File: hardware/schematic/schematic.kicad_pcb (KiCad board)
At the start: 2 copper layers, 23 parts, among them J1 Conn_01x09_Pin, J2 Conn_01x09_Pin, J3 ADS1115, J4 PE_SENSE_1, J5 N_TEST, J6 PE_SENSE_0, J7 PE_FORCE_IN, J8 PE_FORCE_OUT, J9 L_TEST, Q1 Q_NMOS_GSD, U1 LM317

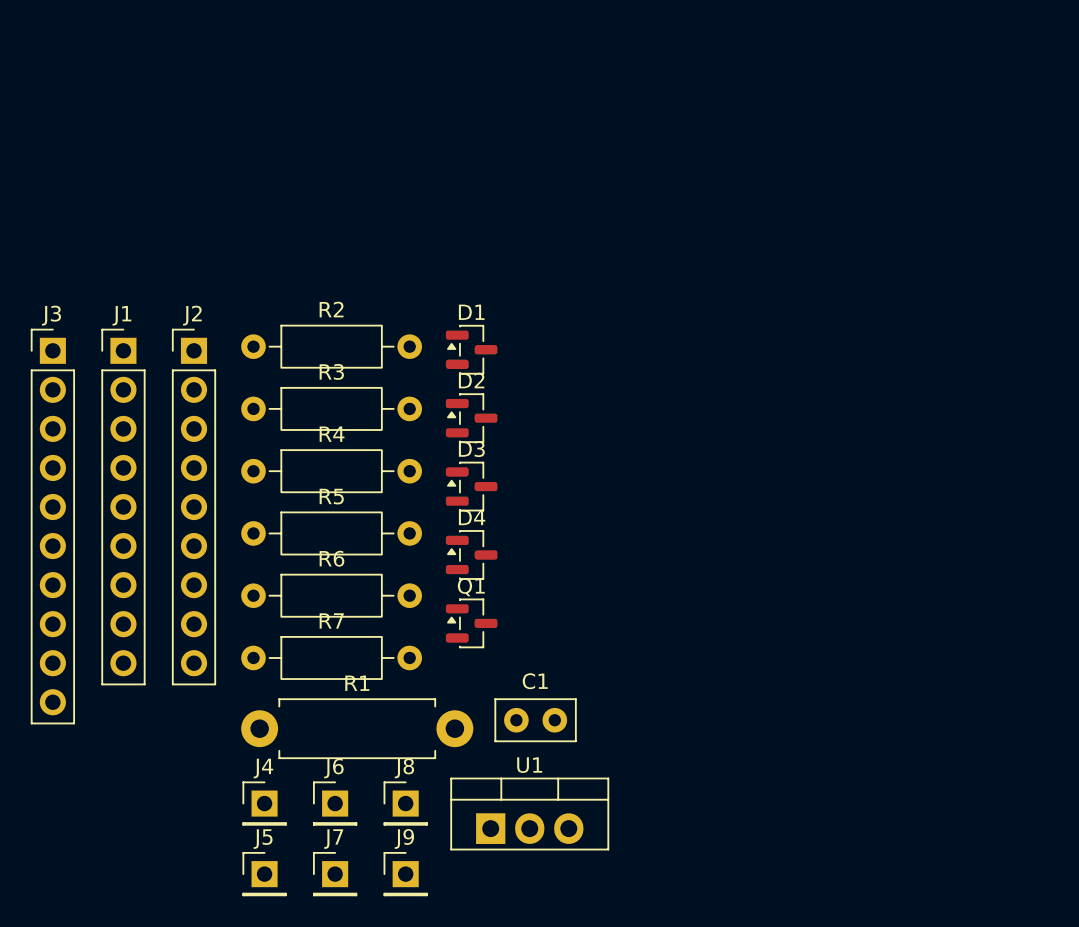
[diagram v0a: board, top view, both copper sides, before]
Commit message: update
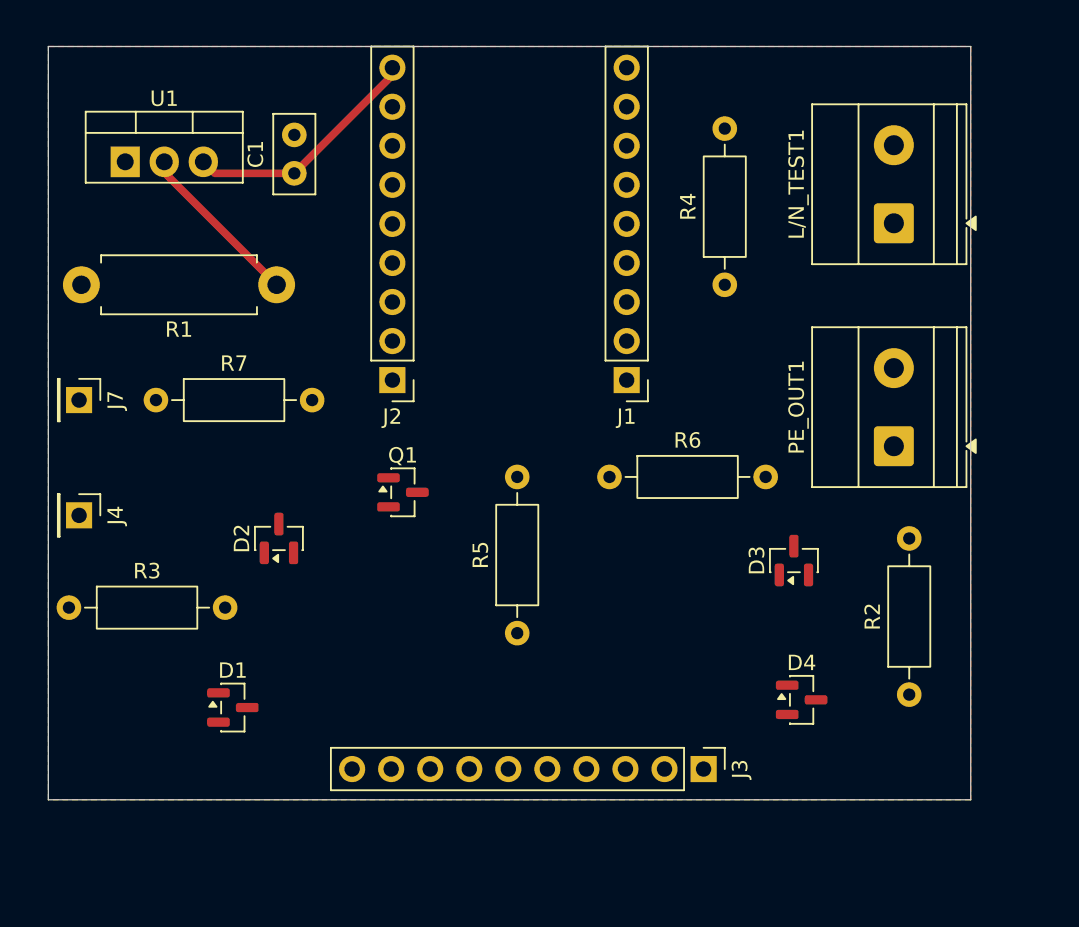
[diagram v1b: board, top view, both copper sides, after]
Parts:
- removed J5: N_TEST, Connector_PinHeader_2.54mm:PinHeader_1x01_P2.54mm_Vertical
- removed J6: PE_SENSE_0, Connector_PinHeader_2.54mm:PinHeader_1x01_P2.54mm_Vertical
- removed J8: PE_FORCE_OUT, Connector_PinHeader_2.54mm:PinHeader_1x01_P2.54mm_Vertical
- removed J9: L_TEST, Connector_PinHeader_2.54mm:PinHeader_1x01_P2.54mm_Vertical
- added L/N_TEST1: Conn_01x02, TerminalBlock_Phoenix:TerminalBlock_Phoenix_MKDS-1,5-2-5.08_1x02_P5.08mm_Horizontal, F.Cu at (142.5, 111.5)
- added PE_OUT1: Conn_01x02, TerminalBlock_Phoenix:TerminalBlock_Phoenix_MKDS-1,5-2-5.08_1x02_P5.08mm_Horizontal, F.Cu at (142.5, 126.0)
- moved J3 50.3 mm to (130.1, 147.0), turned to -90 degrees
- moved U1 49.5 mm to (92.5, 107.5)
- moved R2 48.3 mm to (143.5, 142.2), turned to 90 degrees
- moved C1 38.4 mm to (103.5, 108.2), turned to 90 degrees
- moved J7 35.0 mm to (89.5, 123.0), turned to -90 degrees
- moved R4 33.0 mm to (131.5, 115.5), turned to 90 degrees
- moved J1 32.8 mm to (125.1, 121.7), turned to 180 degrees
- moved R1 28.9 mm to (102.3, 115.5), turned to 180 degrees
- moved D1 28.0 mm to (99.5, 143.0)
- moved R6 24.4 mm to (124.0, 128.0)
- moved D4 23.4 mm to (136.5, 142.5)
- moved J4 22.3 mm to (89.5, 130.5), turned to -90 degrees
- moved D3 21.5 mm to (136.0, 133.4), turned to 90 degrees
- moved R5 18.3 mm to (118.0, 138.2), turned to 90 degrees
- moved R7 17.9 mm to (94.5, 123.0)
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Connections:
- net /<NO NET> renamed +5V
- net Net-(J5-Pin_1) renamed /N_TEST
- J2 pad 8: /GND -> GNDREF
- J3 pad 6: /GND -> GNDREF
- J3 pad 9: /GND -> GNDREF
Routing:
- net +5V: track 0.00 -> 15.7 mm
- net Net-(U1-VO): track 0.00 -> 11.0 mm
- added copper zone on F.Cu, net GNDREF
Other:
- board outline added: 60 x 49 mm

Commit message: update
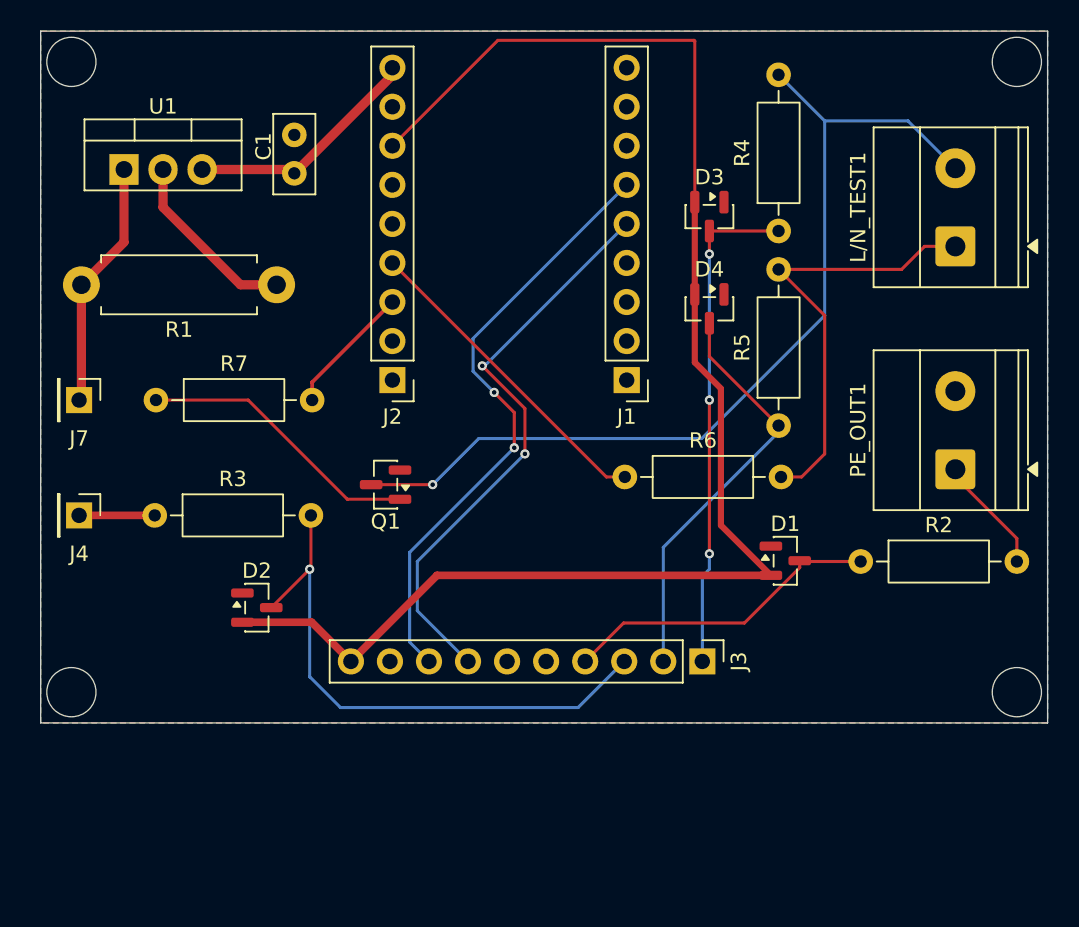
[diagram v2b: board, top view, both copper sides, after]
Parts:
- added REF**: MountingHole_3.2mm_M3, MountingHole:MountingHole_3.2mm_M3, F.Cu at (89.0, 101.0)
- added REF**: MountingHole_3.2mm_M3, MountingHole:MountingHole_3.2mm_M3, F.Cu at (150.5, 101.0)
- added REF**: MountingHole_3.2mm_M3, MountingHole:MountingHole_3.2mm_M3, F.Cu at (89.0, 142.0)
- added REF**: MountingHole_3.2mm_M3, MountingHole:MountingHole_3.2mm_M3, F.Cu at (150.5, 142.0)
- moved D1 37.2 mm to (135.4, 133.4)
- moved D4 26.1 mm to (130.5, 117.1), turned to -90 degrees
- moved D3 23.0 mm to (130.5, 111.1), turned to -90 degrees
- moved R5 21.7 mm to (135.0, 124.7)
- moved R2 9.22 mm to (140.3, 133.5), turned to 0 degrees
- moved R3 8.19 mm to (94.4, 130.5)
- moved J3 7.00 mm to (130.0, 140.0)
- moved R4 4.95 mm to (135.0, 112.0)
- moved D2 4.72 mm to (101.1, 136.5), turned to 0 degrees
- moved L/N_TEST1 4.27 mm to (146.5, 113.0)
- moved PE_OUT1 4.27 mm to (146.5, 127.5)
- moved Q1 1.23 mm to (109.4, 128.5), turned to 180 degrees
- moved R6 1.00 mm to (125.0, 128.0)
- moved U1 0.51 mm to (92.4, 108.0)
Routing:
- net /3V3: track 0.00 -> 97.1 mm
- net /N_TEST: track 0.00 -> 60.7 mm, vias 0 -> 1
- net /I2C_SCL: track 0.00 -> 39.6 mm, vias 0 -> 2
- net /I2C_SDA: track 0.00 -> 37.9 mm, vias 0 -> 2
- net /PE_TEST_RE: track 0.00 -> 36.7 mm, vias 0 -> 1
- net /N_T: track 0.00 -> 32.7 mm, vias 0 -> 3
- net Net-(L/N_TEST1-Pin_1): track 0.00 -> 28.8 mm
- net /L_T: track 0.00 -> 26.6 mm
- net /PE_TEST: track 0.00 -> 20.9 mm
- net /GP27: track 0.00 -> 20.9 mm
- net Net-(Q1-G): track 0.00 -> 18.5 mm
- net Net-(J7-Pin_1): track 0.00 -> 16.2 mm
- net /GP26: track 0.00 -> 8.54 mm
- net Net-(PE_OUT1-Pin_1): track 0.00 -> 7.66 mm
- net Net-(J4-Pin_1): track 0.00 -> 4.92 mm
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- added copper zone on B.Cu, net GNDREF
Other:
- board size 60 x 49 mm -> 65.5 x 45 mm
